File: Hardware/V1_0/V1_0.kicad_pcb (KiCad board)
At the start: 2 copper layers, 73 parts, among them J1 Micro_SD_Card_Det, J10 C, J11 AUDIO, J2 UART5, J3 USB_B_Mini, J4 USART3_UART4, J5 C, J6 C, J7 C, J8 C, J9 C, P1 SWD, U1 LM27762, U2 REF3030, U3 MCP16311_2, U4 STM32F40X_LQFP64, U5 AD5330, U6 LF356, Y1 8M

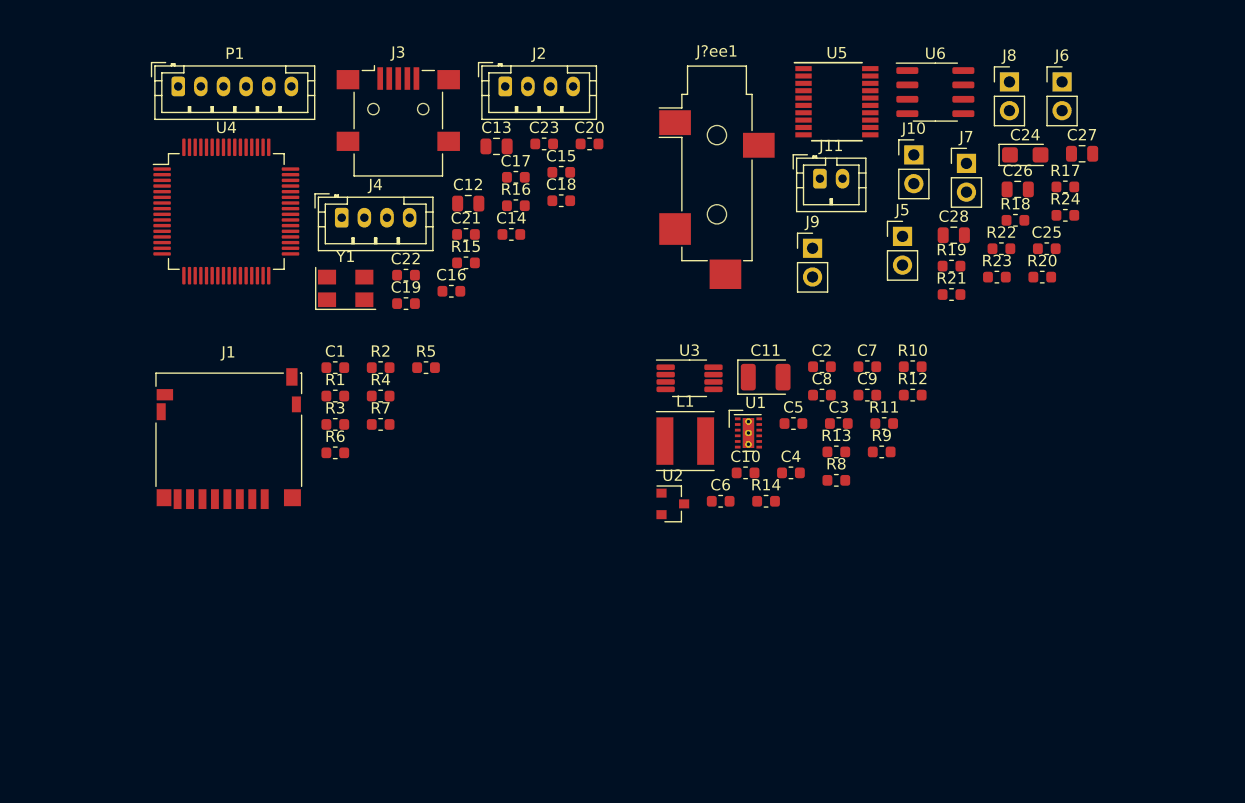
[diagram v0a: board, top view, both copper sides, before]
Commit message: experimenting
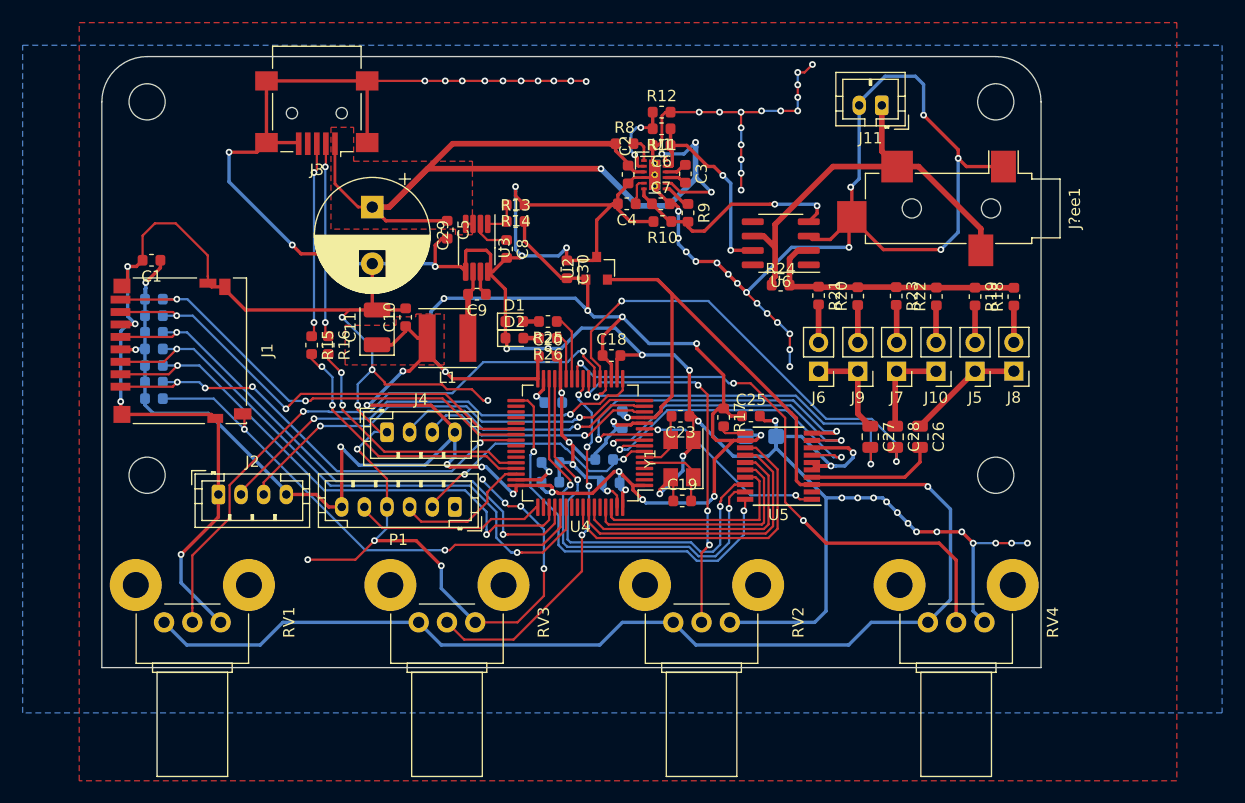
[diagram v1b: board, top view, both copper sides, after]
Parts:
- removed C12, C13: 10uF, Capacitor_SMD:C_0805_2012Metric
- added C29: 100u, Capacitor_THT:CP_Radial_D10.0mm_P5.00mm, F.Cu at (122.9, 93.3)
- added C30: 2.2u, Capacitor_SMD:C_0603_1608Metric, F.Cu at (140.1, 98.8)
- added D1: RED, LED_SMD:LED_0603_1608Metric, F.Cu at (135.4, 103.4)
- added D2: GREEN, LED_SMD:LED_0603_1608Metric, F.Cu at (135.5, 104.9)
- added MK1: Mounting_Hole, MountingHole:MountingHole_3.2mm_M3, F.Cu at (178.0, 117.0)
- added MK2: Mounting_Hole, MountingHole:MountingHole_3.2mm_M3, F.Cu at (178.0, 84.0)
- added MK3: Mounting_Hole, MountingHole:MountingHole_3.2mm_M3, F.Cu at (103.0, 84.0)
- added MK4: Mounting_Hole, MountingHole:MountingHole_3.2mm_M3, F.Cu at (103.0, 117.0)
- added R25: 1k, Resistor_SMD:R_0603_1608Metric, F.Cu at (138.4, 103.4)
- added R26: 1k, Resistor_SMD:R_0603_1608Metric, F.Cu at (138.4, 104.9)
- added RV1: R_POT, Potentiometer_THT:Potentiometer_Bourns_PTV09A-2_Single_Horizontal, F.Cu at (104.5, 130.0)
- added RV2: R_POT, Potentiometer_THT:Potentiometer_Bourns_PTV09A-2_Single_Horizontal, F.Cu at (149.5, 130.0)
- added RV3: R_POT, Potentiometer_THT:Potentiometer_Bourns_PTV09A-2_Single_Horizontal, F.Cu at (127.0, 130.0)
- added RV4: R_POT, Potentiometer_THT:Potentiometer_Bourns_PTV09A-2_Single_Horizontal, F.Cu at (172.0, 130.0)
- C14, C15, C16, C17, C21, C22, C24, R1, R2, R3, R4, R5, R6, R7: moved to B.Cu
- J2: value UART5 -> USART2
- J4: value USART3_UART4 -> UART
- moved P1 44.5 mm to (130.2, 119.8), turned to 180 degrees
- moved J2 44.1 mm to (109.3, 118.7)
- moved U4 37.4 mm to (141.3, 114.2), turned to 180 degrees
- moved R17 36.4 mm to (153.9, 111.9), turned to -90 degrees
- moved C9 35.6 mm to (132.2, 101.0), turned to 180 degrees
- moved R8 35.1 mm to (145.2, 87.7)
- moved C5 35.1 mm to (129.5, 95.3), turned to -90 degrees
- moved R13 34.9 mm to (135.6, 94.6)
- moved C11 34.6 mm to (123.3, 103.9), turned to 90 degrees
- moved R14 34.3 mm to (135.6, 93.1), turned to 180 degrees
- moved C24 34.1 mm to (157.2, 113.6)
- moved R12 33.4 mm to (148.5, 84.9)
- moved J6 33.4 mm to (162.3, 107.8), turned to 180 degrees
- moved Y1 33.3 mm to (150.3, 115.5), turned to 90 degrees
- moved C10 33.0 mm to (125.8, 103.0), turned to 90 degrees
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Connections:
- J2 pad 2: /MCU/UART5_RX -> /MCU/USART2_RX
- J2 pad 3: /MCU/UART5_TX -> /MCU/USART2_TX
- U4 pad 14: Net-(U4-Pad14) -> /MCU/UART_TXD
- U4 pad 15: Net-(U4-Pad15) -> /MCU/UART_RXD
- U4 pad 16: Net-(U4-Pad16) -> /MCU/USART2_TX
- U4 pad 17: Net-(U4-Pad17) -> /MCU/USART2_RX
- U4 pad 20: Net-(C13-Pad1) -> /DAC1
- U4 pad 21: Net-(C12-Pad1) -> /DAC2
- U4 pad 22: Net-(U4-Pad22) -> /MCU/POT1
- U4 pad 23: Net-(U4-Pad23) -> /MCU/POT2
- U4 pad 24: Net-(U4-Pad24) -> /MCU/POT3
- U4 pad 25: Net-(U4-Pad25) -> /MCU/POT4
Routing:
- net GND: track 0.00 -> 569.7 mm, vias 0 -> 95
- net +3V3: track 0.00 -> 202.1 mm, vias 0 -> 19
- net /VREF: track 0.00 -> 142.0 mm, vias 0 -> 2
- net +5V: track 0.00 -> 88.0 mm, vias 0 -> 4
- net /SDIO_CMD: track 0.00 -> 52.7 mm, vias 0 -> 2
- net /MCU/POT1: track 0.00 -> 52.6 mm, vias 0 -> 2
- net /MCU/POT4: track 0.00 -> 51.8 mm, vias 0 -> 3
- net /SDIO_CK: track 0.00 -> 50.2 mm, vias 0 -> 2
- net /SDIO_D3: track 0.00 -> 48.5 mm, vias 0 -> 2
- net /SDIO_DET: track 0.00 -> 44.7 mm, vias 0 -> 2
- net /SDIO_D0: track 0.00 -> 41.6 mm, vias 0 -> 2
- net /SDIO_D1: track 0.00 -> 41.3 mm, vias 0 -> 2
- net /SDIO_D2: track 0.00 -> 40.9 mm, vias 0 -> 4
- net /DAC2: track 0.00 -> 40.7 mm, vias 0 -> 2
- net /MCU/USART2_RX: track 0.00 -> 40.0 mm, vias 0 -> 2
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- added copper zone on F.Cu, net +3V3
- added copper zone on F.Cu, net +5V
- added copper zone on B.Cu, net GND
- added copper zone on F.Cu, net GND
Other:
- board outline added: 83 x 54 mm
- rule pad_to_mask_clearance: 0.051 -> 0.01
- rule solder_mask_min_width: 0.25 -> 0.025
- rule trace_min: 0.2 -> 0.18
